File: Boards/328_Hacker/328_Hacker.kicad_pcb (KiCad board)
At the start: 2 copper layers, 35.6 x 58.4 mm, 18 parts, among them J1 Conn_01x11, J2 Conn_01x11, J3 CONN_02X03, J4 CONN_02X03, J5 Conn_02x02, U1 ATmega328P-AU, Y1 Crystal_SMD

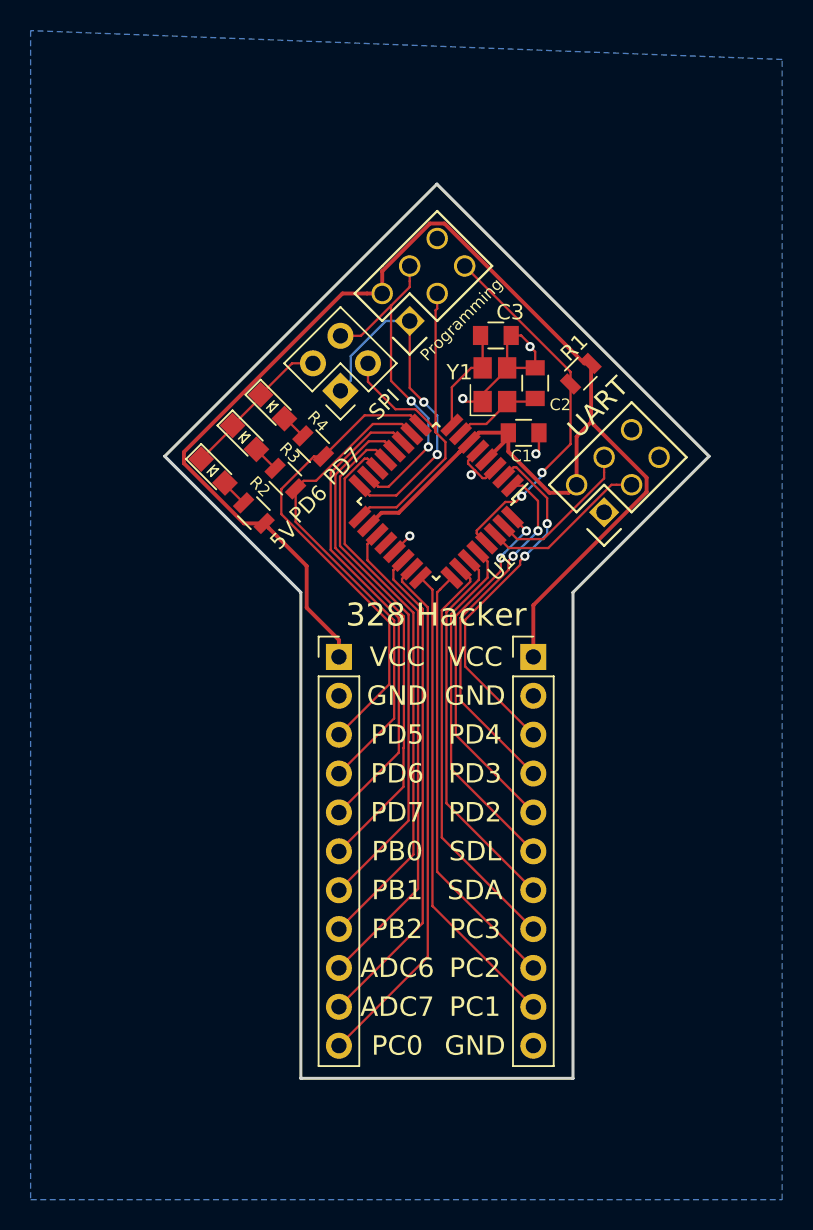
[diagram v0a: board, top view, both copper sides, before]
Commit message: Addressed review comments
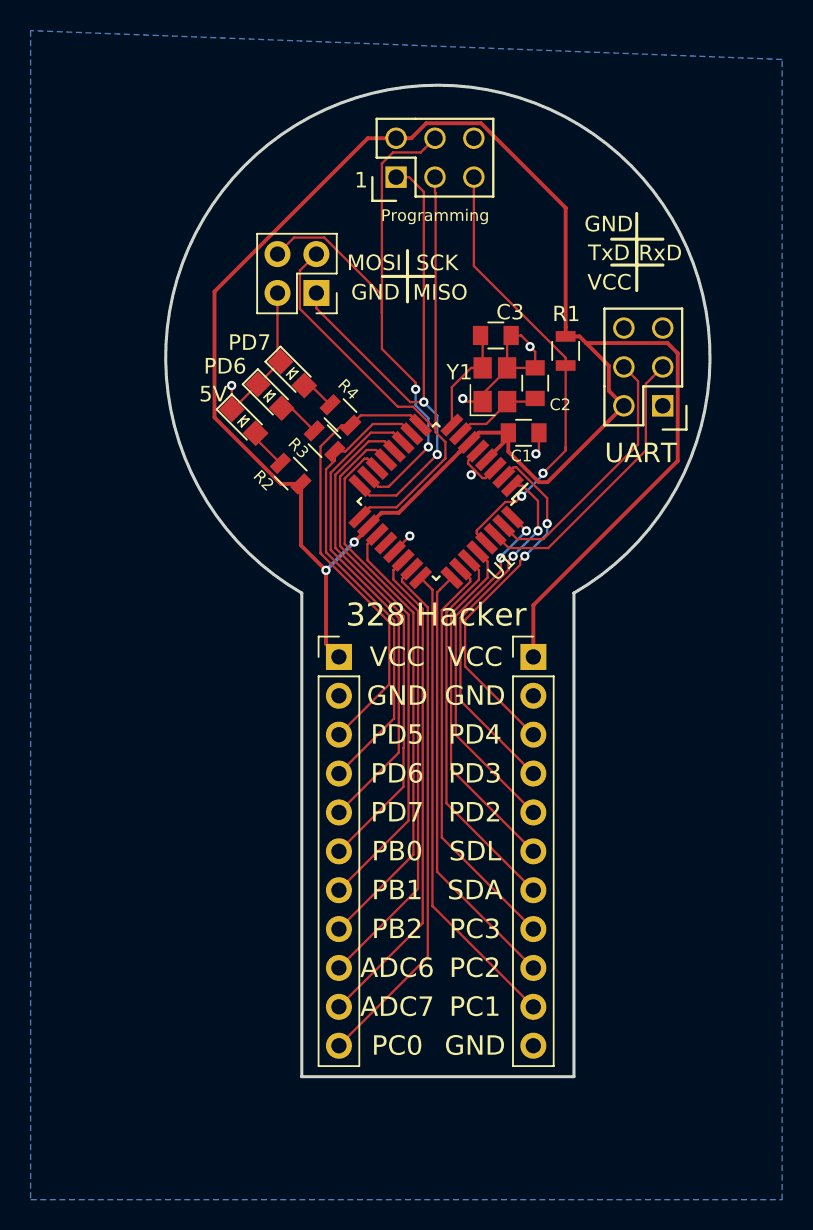
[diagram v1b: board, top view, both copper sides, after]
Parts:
- moved J4 9.44 mm to (67.2, 29.6), turned to 90 degrees
- moved J3 7.94 mm to (84.7, 44.6), turned to 180 degrees
- moved J5 6.58 mm to (62.0, 37.2), turned to 270 degrees
- moved D1 3.81 mm to (57.3, 45.6)
- moved R3 3.54 mm to (62.6, 46.9)
- moved R2 3.53 mm to (60.4, 49.0)
- moved D2 3.16 mm to (59.0, 43.9)
- moved R4 2.71 mm to (63.6, 45.2)
- moved D3 2.52 mm to (60.5, 42.5)
- moved R1 1.79 mm to (78.3, 41.0), turned to 270 degrees
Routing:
- net VCC: track 105.1 -> 132.9 mm, vias 0 -> 2
- net /SCK: track 25.4 -> 42.0 mm
- net /MOSI: track 22.7 -> 39.2 mm
- net /MISO: track 23.2 -> 36.7 mm
- net /RxD: track 11.0 -> 18.8 mm
- net /TxD: track 9.93 -> 17.1 mm
- net /~RESET: track 24.2 -> 29.6 mm
- net /1L: track 31.7 -> 29.7 mm
- net /2L: track 32.4 -> 30.7 mm
- net Net-(D2-Pad2): track 1.75 -> 2.75 mm
- net Net-(D1-Pad2): track 1.81 -> 2.64 mm
- net Net-(D3-Pad2): track 1.67 -> 2.21 mm
- net GND: track 28.3 -> 28.9 mm, vias 5 -> 6
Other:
- board size 35.6 x 58.4 mm -> 35.6 x 64.8 mm
- board text added: "1"
- board text added: "MISO"
- board text added: "MOSI"
- board text added: "RxD"
- board text added: "SCK"
- board text added: "TxD"
- board text removed: "SPI"
